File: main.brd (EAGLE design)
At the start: 146.5 x 85 mm, 53 parts, among them X1 ZX62D-B-5PA8

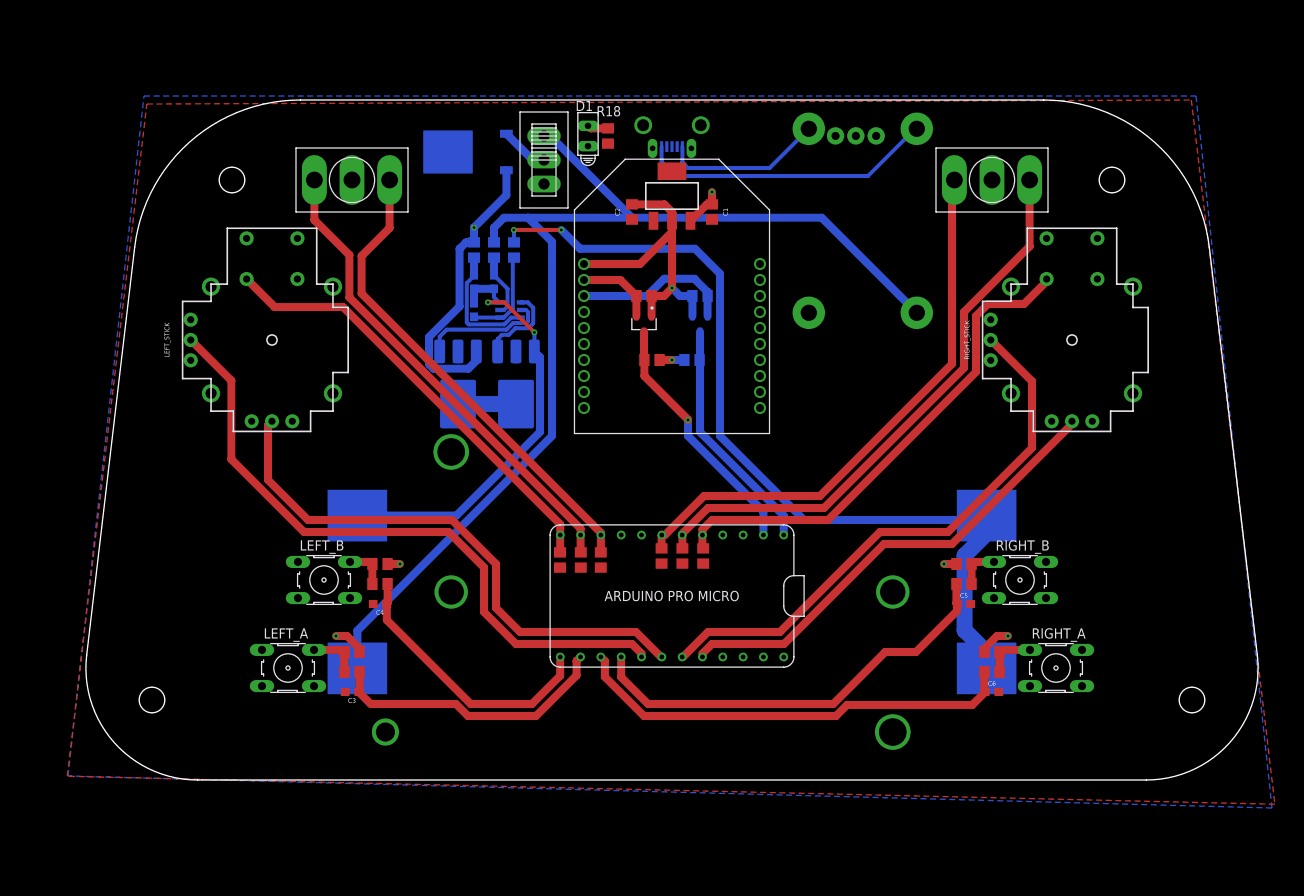
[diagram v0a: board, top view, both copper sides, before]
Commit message: Incorporated Feedback
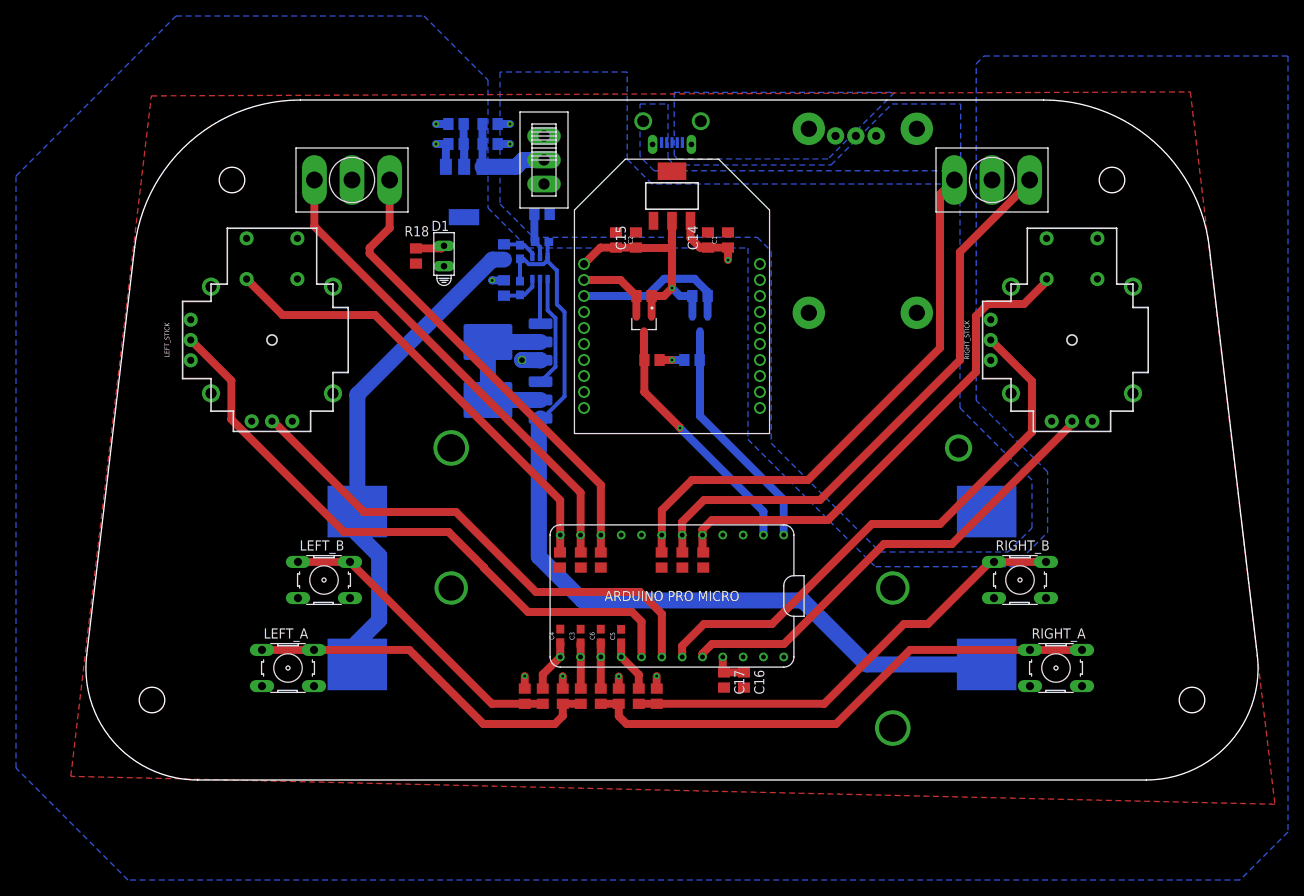
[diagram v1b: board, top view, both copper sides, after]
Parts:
- removed U$5: NCV7805, CustomParts:TO-252
- added C10, C11, C15, C17: 0.1uF, rcl:C0805
- added C12: 10uF, rcl:C0805
- added C13: 22uF, rcl:C0805
- added C14: 100nF, rcl:C0805
- added C16: 47uF, rcl:C0805
- added IC1: REG1117, burr-brown:SOT223
- C1: value 0.1uF -> 10uF
- C2: value 0.1uF -> 22uF
- moved C6 49.4 mm to (-8.91, -25.5), turned to 90 degrees
- moved R8 49.0 mm to (-8.91, -33.0), turned to 270 degrees
- moved R7 47.0 mm to (-6.66, -33.0), turned to 90 degrees
- moved C5 43.0 mm to (-6.36, -25.5), turned to 90 degrees
- moved R6 43.0 mm to (-4.16, -33.0), turned to 270 degrees
- moved R5 41.8 mm to (-1.91, -33.0), turned to 90 degrees
- moved C3 29.4 mm to (-11.4, -25.5), turned to 90 degrees
- moved R2 28.8 mm to (-11.4, -33.0), turned to 270 degrees
- moved R18 28.3 mm to (-32.0, 22.0)
- moved R1 26.9 mm to (-13.7, -33.0), turned to 90 degrees
- moved R4 24.7 mm to (-16.2, -33.0), turned to 270 degrees
- moved R3 24.5 mm to (-18.4, -33.0), turned to 90 degrees
- moved D1 23.4 mm to (-28.5, 22.0)
- moved C4 22.9 mm to (-14.0, -25.5), turned to 90 degrees
- moved C8 9.25 mm to (-19.0, 22.5), turned to 270 degrees
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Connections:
- net N$1 renamed P+
- net N$2 renamed P-
- removed net N$4: U$5.1, U$6.2
- new net 8V4_IN: C10.1, C12.1, IC1.3, U$6.2
- net 3V3: now also C15.1
- net GND: now also C10.2, C11.2, C12.2, C13.2, C14.2, C15.2, C16.2, C17.2, IC1.1, LEFT_A.3, LEFT_B.3, RIGHT_A.4, RIGHT_B.4; no longer U$5.2
- net LEFT_A_SW: now also LEFT_A.1
- net LEFT_B_SW: now also LEFT_B.1
- net RIGHT_A_SW: now also RIGHT_A.2
- net RIGHT_B_SW: now also RIGHT_B.2
- net VCC: now also C11.1, C13.1, C14.1, C16.1, C17.1, IC1.2; no longer U$5.3
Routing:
- net B+: track 143.0 -> 0.00 mm
- net RIGHT_A_SW: track 6.41 -> 65.9 mm
- net VSS: track 54.9 -> 110.5 mm, vias 2 -> 0
- net RIGHT_B_SW: track 5.41 -> 58.3 mm
- net RIGHT_A: track 56.0 -> 5.76 mm
- net RIGHT_B: track 54.1 -> 6.62 mm
- net BM: track 108.8 -> 61.4 mm, vias 2 -> 0
- net LEFT_A_SW: track 6.41 -> 45.6 mm
- net P+: track 37.0 -> 0.00 mm
- net LEFT_B_SW: track 5.41 -> 37.9 mm
- net LEFT_A: track 35.6 -> 5.73 mm
- net LEFT_B: track 34.4 -> 6.65 mm
- net GND: track 36.7 -> 13.0 mm, vias 1 -> 6
- net P-: track 20.1 -> 0.00 mm
- net 8V4_IN: track 0.00 -> 13.4 mm
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- added copper zone on layer 16, net B+
- added copper zone on layer 16, net P+
- added copper zone on layer 16, net P-
